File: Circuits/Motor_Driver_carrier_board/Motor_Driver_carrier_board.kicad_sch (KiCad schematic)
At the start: 2 parts, among them P2 61301021021

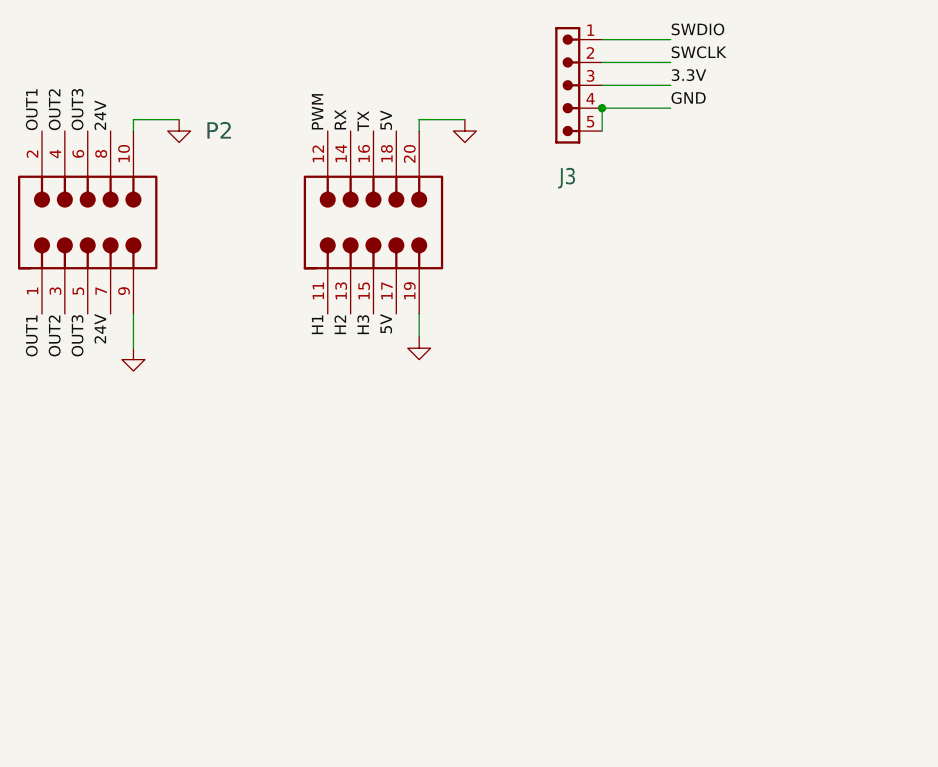
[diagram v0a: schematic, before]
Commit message: STP to pointer
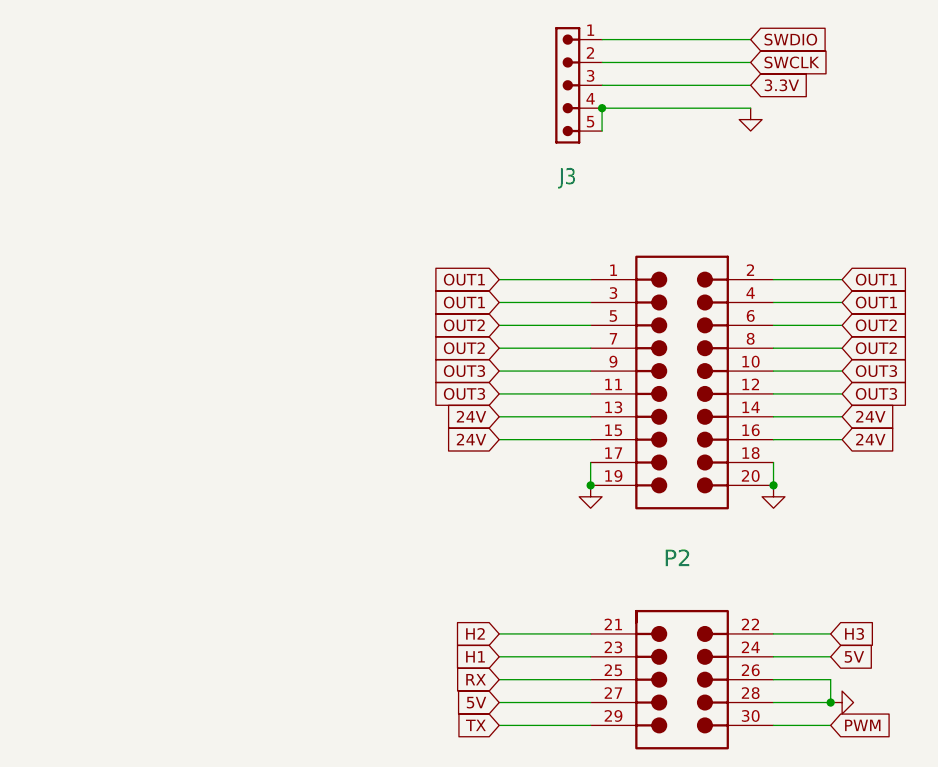
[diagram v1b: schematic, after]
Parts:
- P2: value 61301021021 -> ESC_Adapter_pins_right_angle; footprint 61301021021:ESC_Adapter_pins_right_angle -> B-G431B-ESC1:ESC_Adapter_pins_right_angle
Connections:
- net 24V: now also P2.13, P2.14, P2.15, P2.16; no longer P2.7, P2.8
- net 5V: now also P2.24, P2.27; no longer P2.17, P2.18
- net GND: now also P2.17, P2.18, P2.26, P2.28; no longer P2.10, P2.9
- net H1: now also P2.23; no longer P2.11
- net H2: now also P2.21; no longer P2.13
- net H3: now also P2.22; no longer P2.15
- net OUT1: now also P2.3, P2.4
- net OUT2: now also P2.5, P2.6, P2.7, P2.8; no longer P2.3, P2.4
- net OUT3: now also P2.10, P2.11, P2.12, P2.9; no longer P2.5, P2.6
- net PWM: now also P2.30; no longer P2.12
- net RX: now also P2.25; no longer P2.14
- net TX: now also P2.29; no longer P2.16
